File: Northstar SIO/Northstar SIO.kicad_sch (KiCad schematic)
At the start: 50 parts, among them J1 DB25_Female, J1A1 Clock Header, J2 Conn_02x15_Odd_Even, J3A1 Configuration Header, U1B1 74LS161, U1C1 74LS161, U1D1 74LS161, U1E1 74LS174, U2A1 MC1489PG, U2B1 74LS04, U2C1 74LS109, U2D1 74LS175, U2E1 74LS243, U3B1 74LS00, U3C1 74LS138, U3D1 74LS03, U3E1 74LS243, U4A1 MC1488N, U4E1 8251A

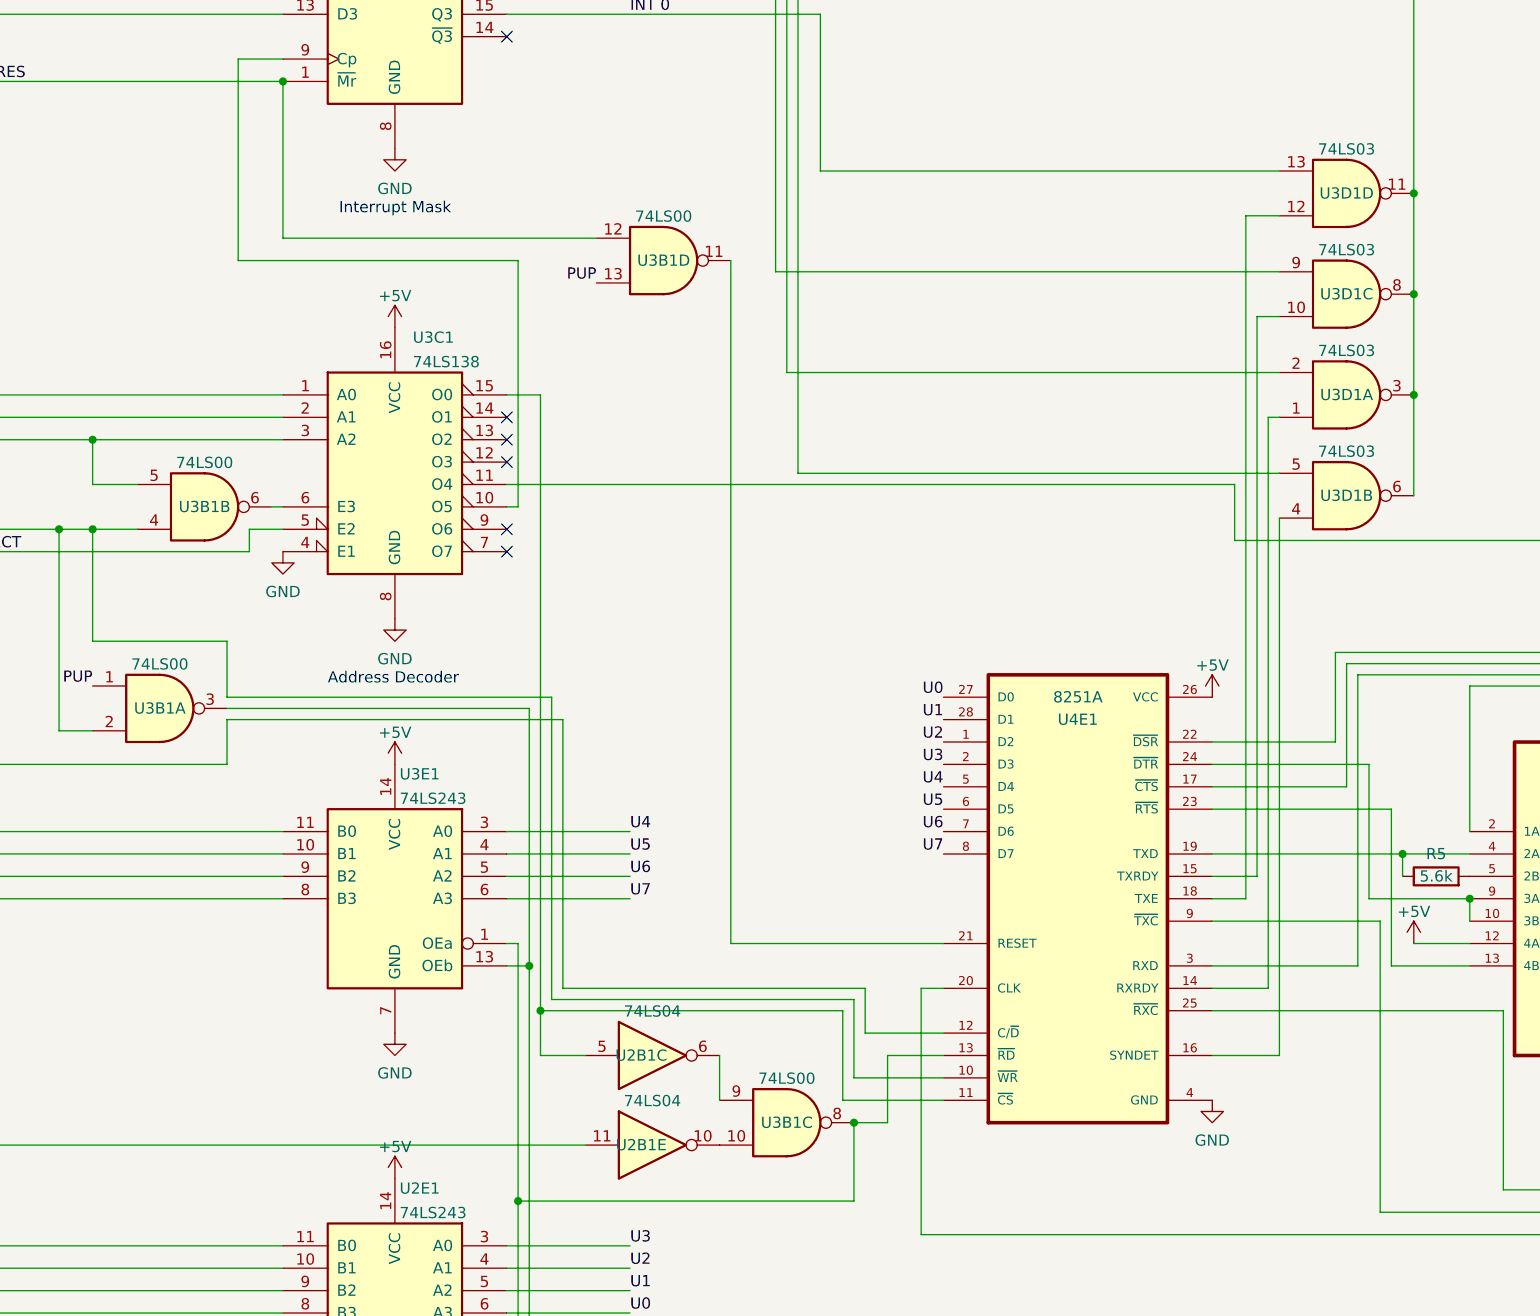
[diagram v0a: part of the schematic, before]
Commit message: small updates to boards
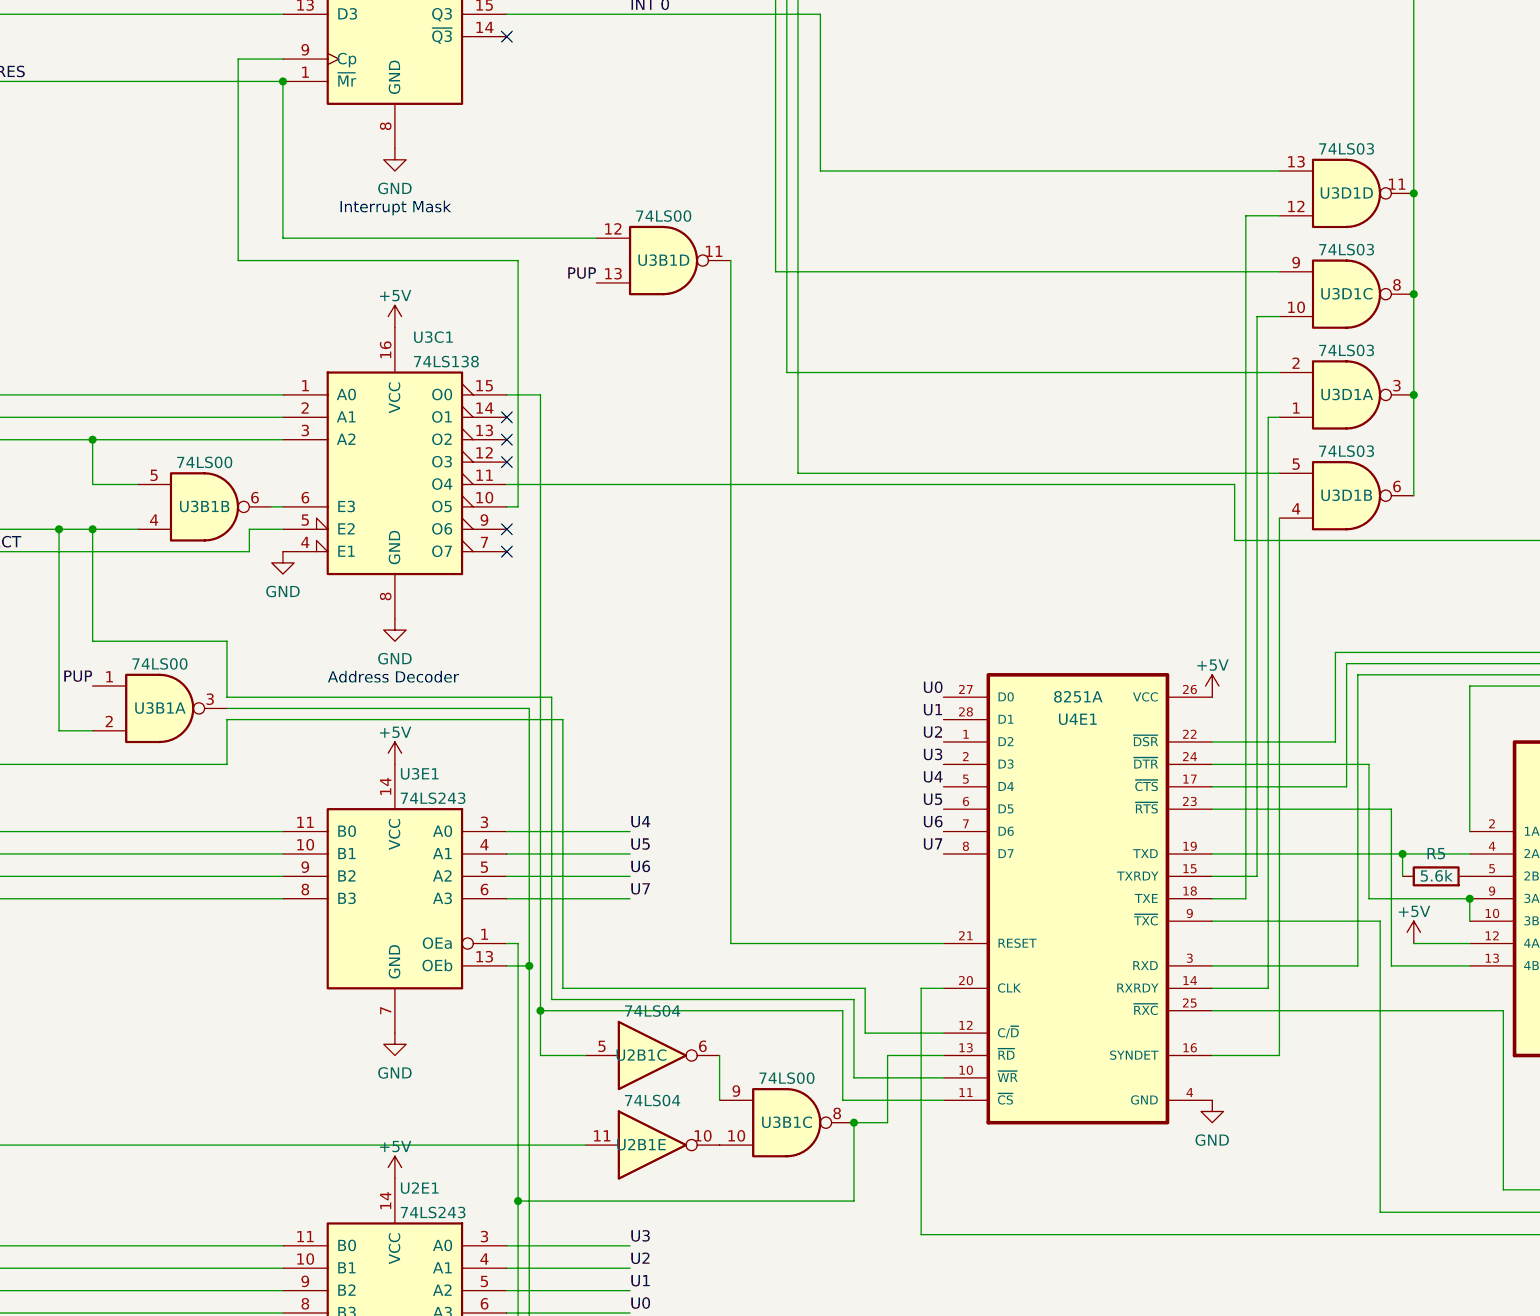
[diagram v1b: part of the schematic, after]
